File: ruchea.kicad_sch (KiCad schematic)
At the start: 25 parts, among them J11 Conn_01x04, J12 Conn_01x04, J14 Conn_01x03, J17 Conn_01x04, J18 Conn_01x04, J3 Conn_01x03, J4 Conn_01x03, J5 Conn_01x04, J6 Conn_01x02, J7 Conn_01x02, J8 Conn_01x03, J9 Conn_01x03, U4 TCA9548APWR

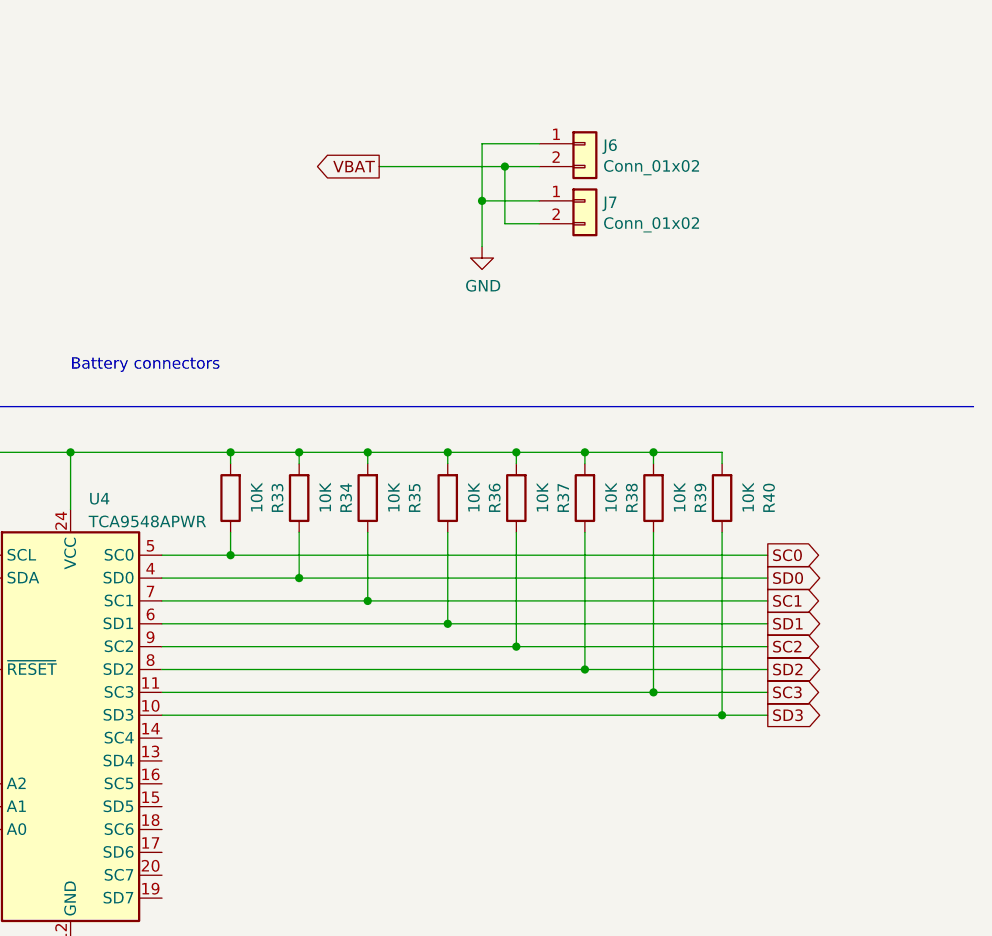
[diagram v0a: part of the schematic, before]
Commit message: update
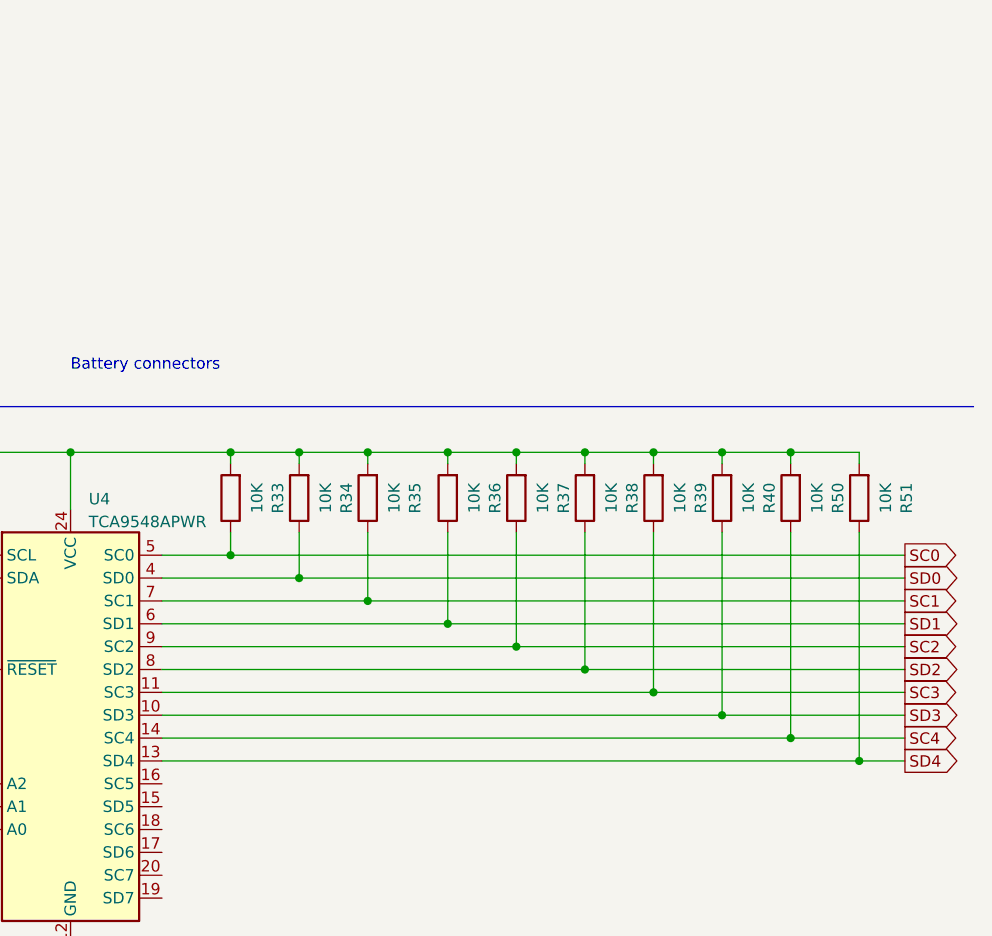
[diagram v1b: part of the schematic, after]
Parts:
- removed J6, J7: Conn_01x02, Connector_JST:JST_PH_B2B-PH-K_1x02_P2.00mm_Vertical, symbol Connector_Generic:Conn_01x02
- added R50, R51: 10K, Resistor_SMD:R_0603_1608Metric, symbol Device:R
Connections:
- net VCC: now also R50.2, R51.2
- net SD4: now reaches U4.13 (SD4)
- net SD4: now also R51.1
- net SC4: now reaches U4.14 (SC4)
- net SC4: now also R50.1
